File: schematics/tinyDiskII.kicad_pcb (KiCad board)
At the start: 2 copper layers, 95.3 x 50.8 mm, 51 parts, among them J2 SD_Card, J3 USB_B_Mini, J4 APPLEII_DISK_CONNECTOR, J5 Ext, SW1 RotaryEncoder_Switch, U1 MX25R3235FM1xx0, U10 AP1117-33, U2 SN74LVC244, U3 CH340C, U5 74LS125, U7 OLED_MULTI

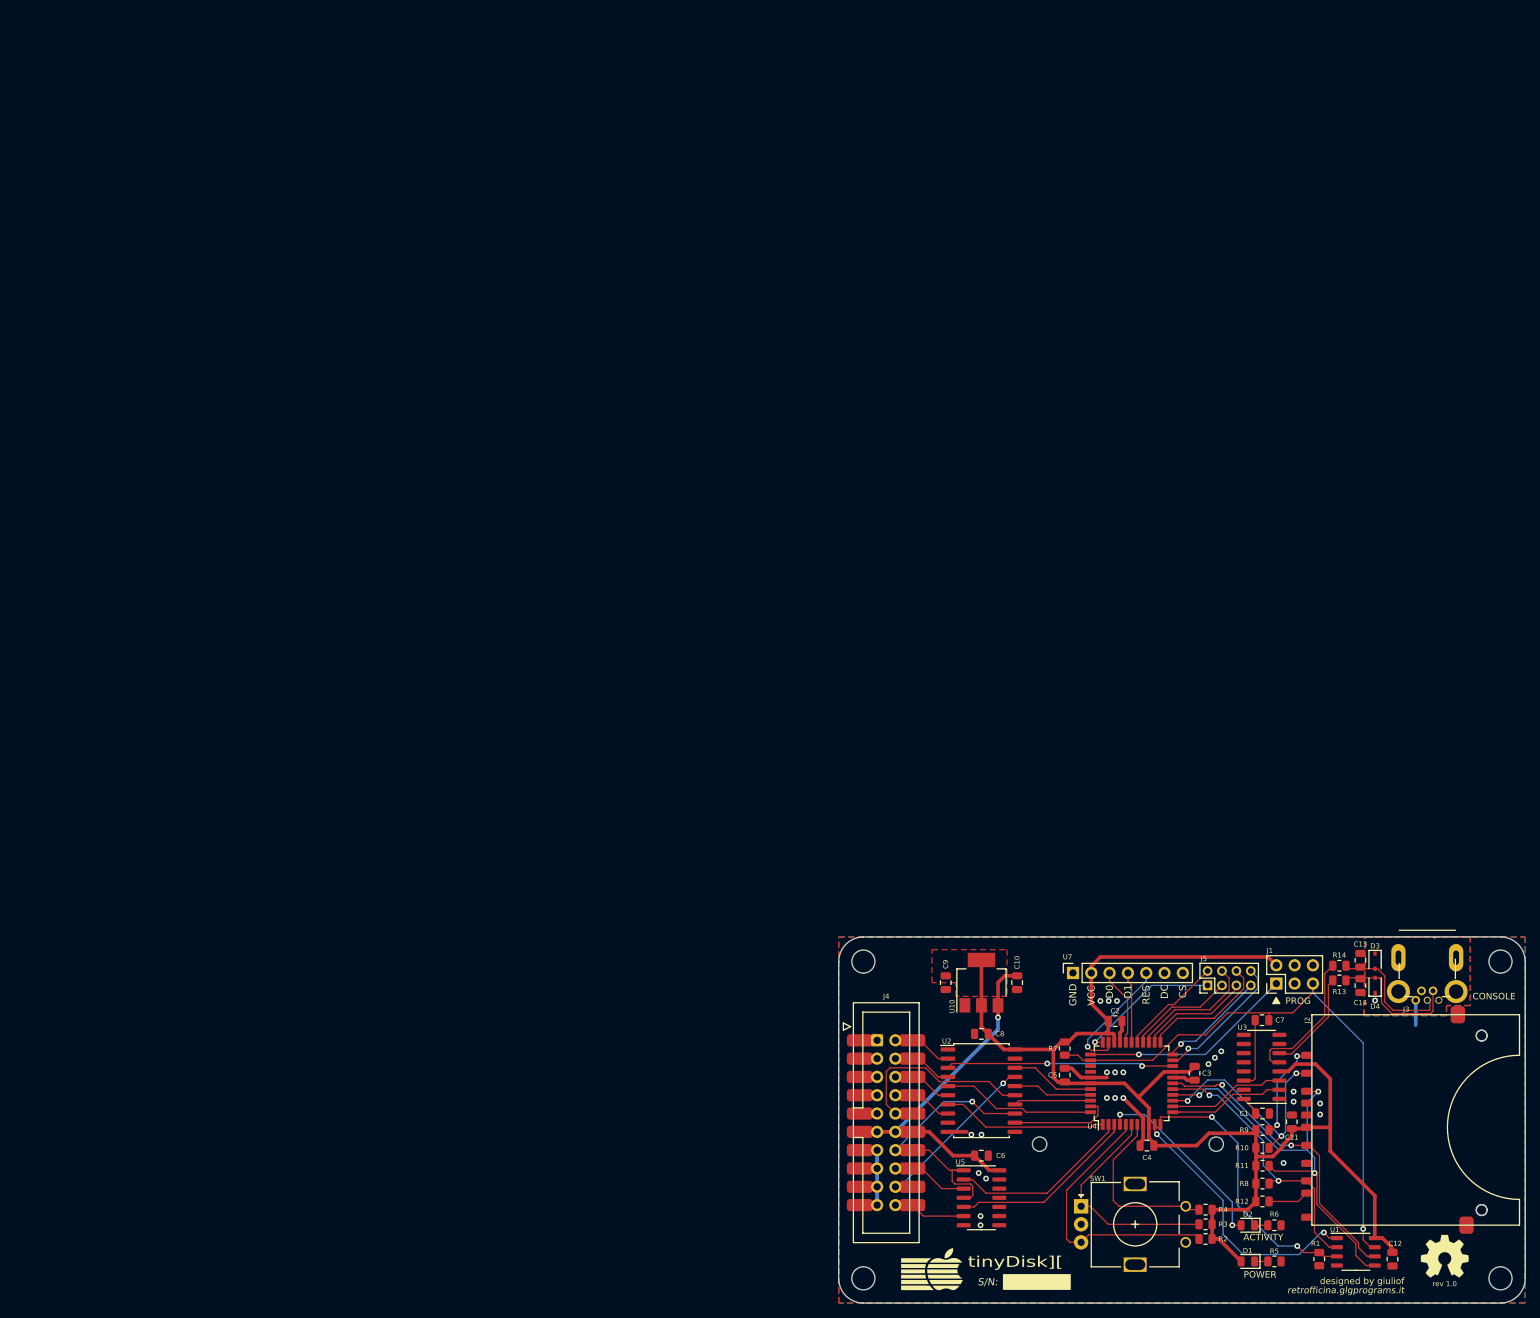
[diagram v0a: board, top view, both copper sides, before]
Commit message: Annotations for next release
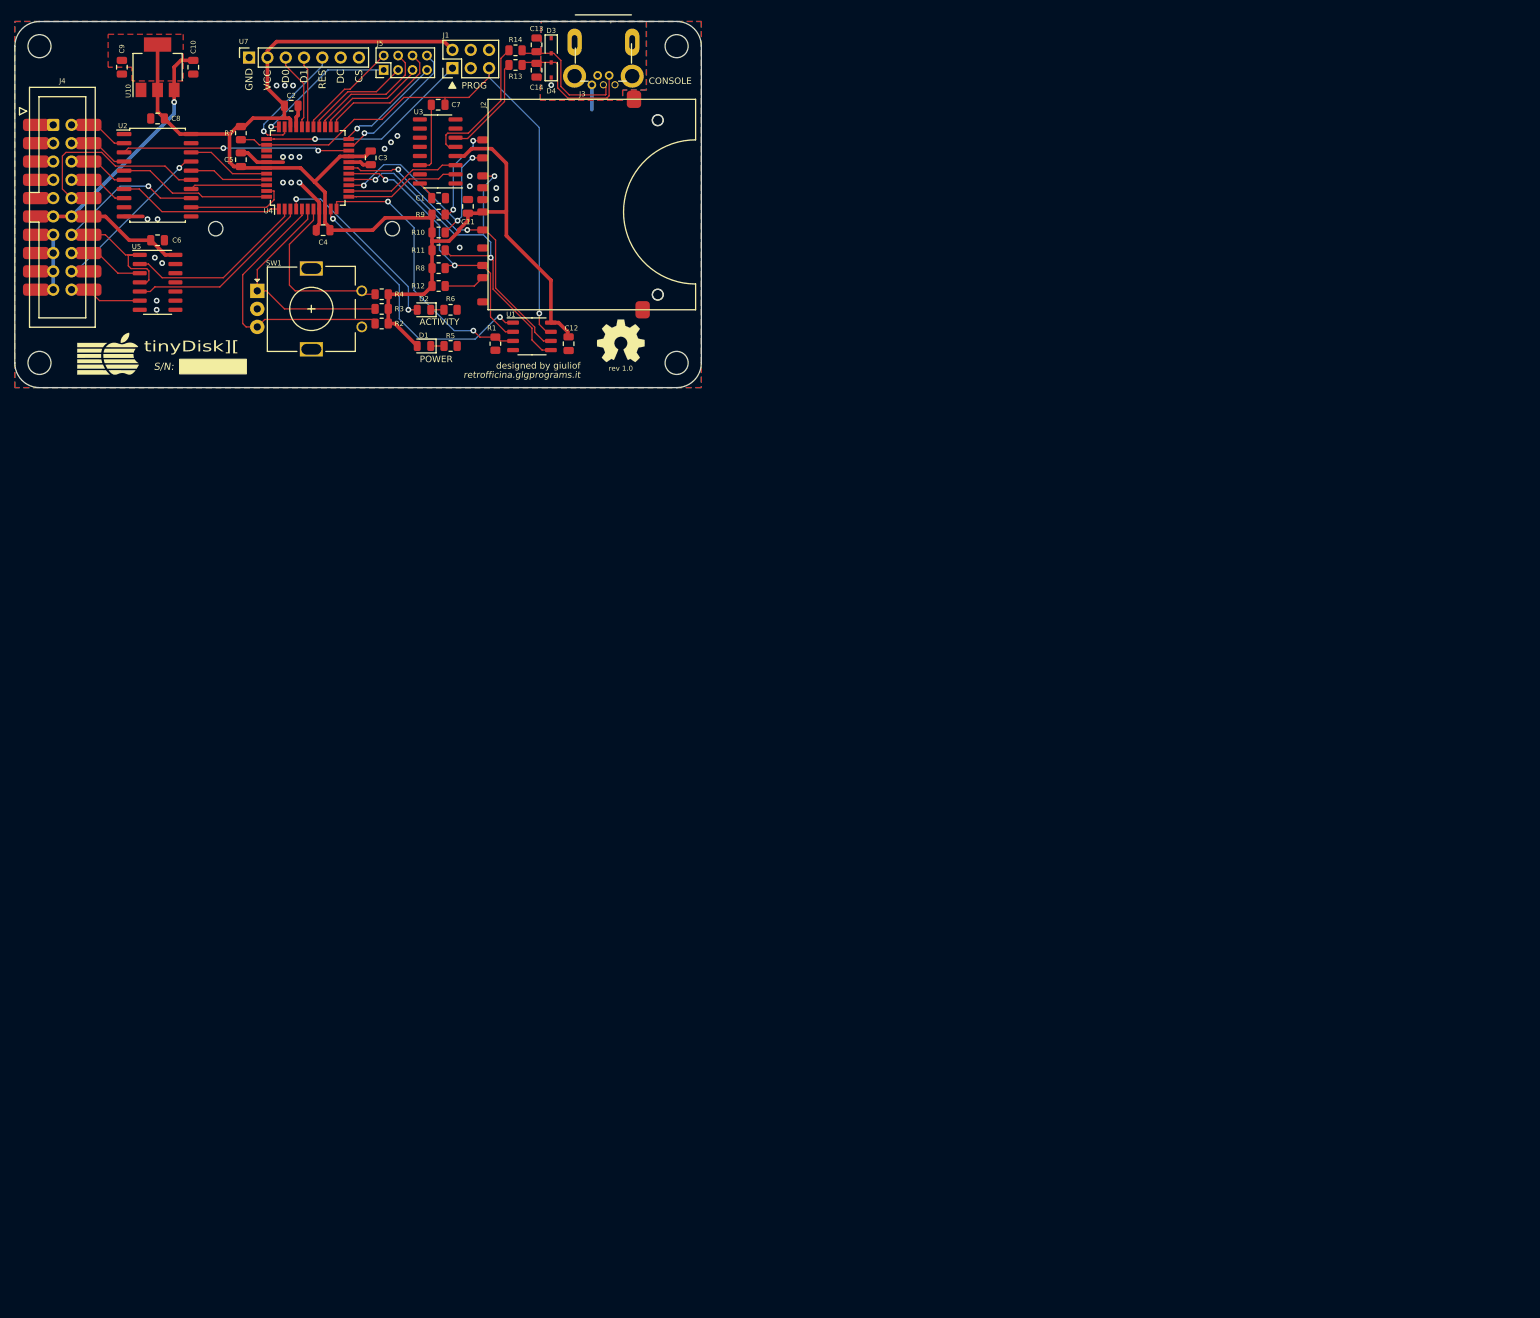
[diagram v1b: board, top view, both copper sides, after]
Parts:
- moved C1 170.9 mm to (58.8, -26.3)
- moved C10 170.9 mm to (24.8, -44.5)
- moved C12 170.9 mm to (76.8, -6.10)
- moved C13 170.9 mm to (72.4, -47.6)
- moved C14 170.9 mm to (72.4, -44.0)
- moved C3 170.9 mm to (49.4, -31.9)
- moved C5 170.9 mm to (31.4, -31.6)
- moved C6 170.9 mm to (19.8, -20.4)
- moved C7 170.9 mm to (58.7, -39.2)
- moved C8 170.9 mm to (19.8, -37.3)
- moved C9 170.9 mm to (14.9, -44.5)
- moved C? 170.9 mm to (38.4, -39.1)
- moved D1 170.9 mm to (56.8, -5.78)
- moved D3 170.9 mm to (74.4, -47.4)
- moved D4 170.9 mm to (74.4, -44.1)
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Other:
- board size 95.3 x 50.8 mm -> 95.2 x 50.8 mm
